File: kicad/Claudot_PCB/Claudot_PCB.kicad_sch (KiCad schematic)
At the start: 27 parts, among them SW1 SW_Push, SW10 SW_Push, SW11 SW_Push, SW12 RotaryEncoder, SW2 SW_Push, SW3 SW_Push, SW4 SW_Push, SW5 SW_Push, SW6 SW_Push, SW7 SW_Push, SW8 SW_Push, SW9 SW_Push, U1 AP2112K-3.3, U2 W25Q16JVUXIQ, U3 RP2040, Y1 Crystal_GND24

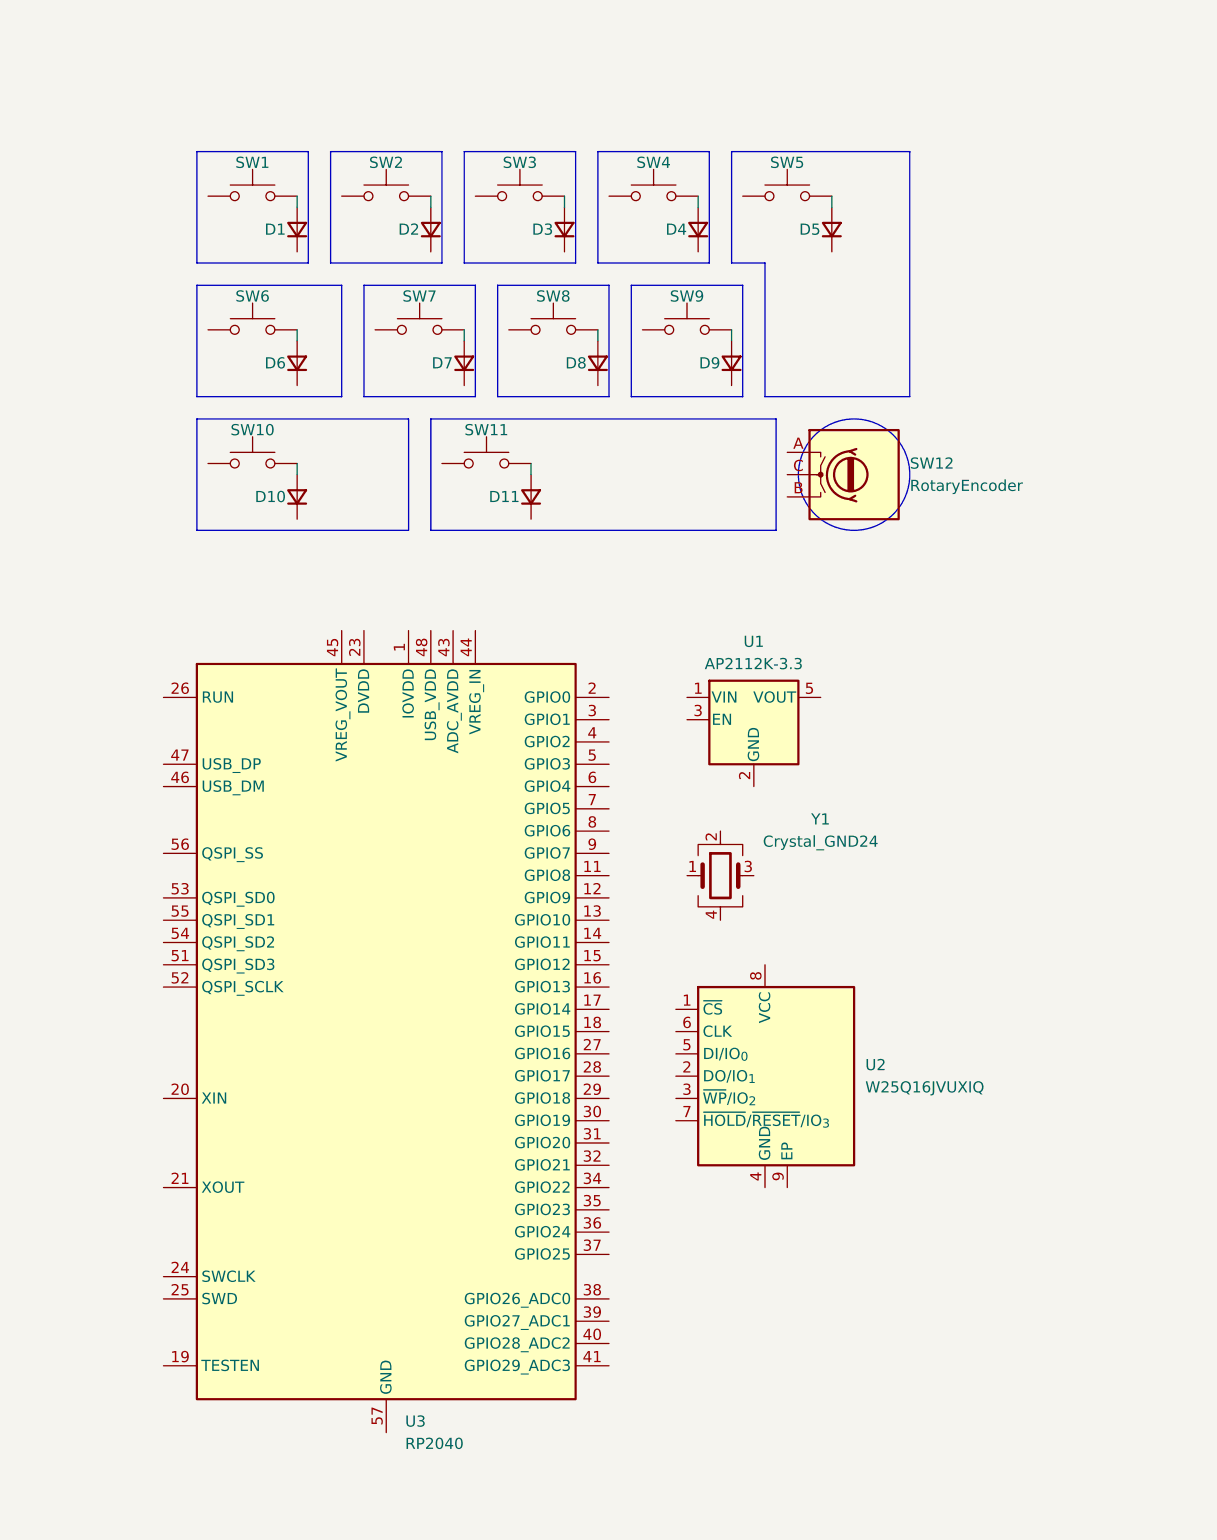
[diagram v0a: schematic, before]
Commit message: Update schematic and pcb
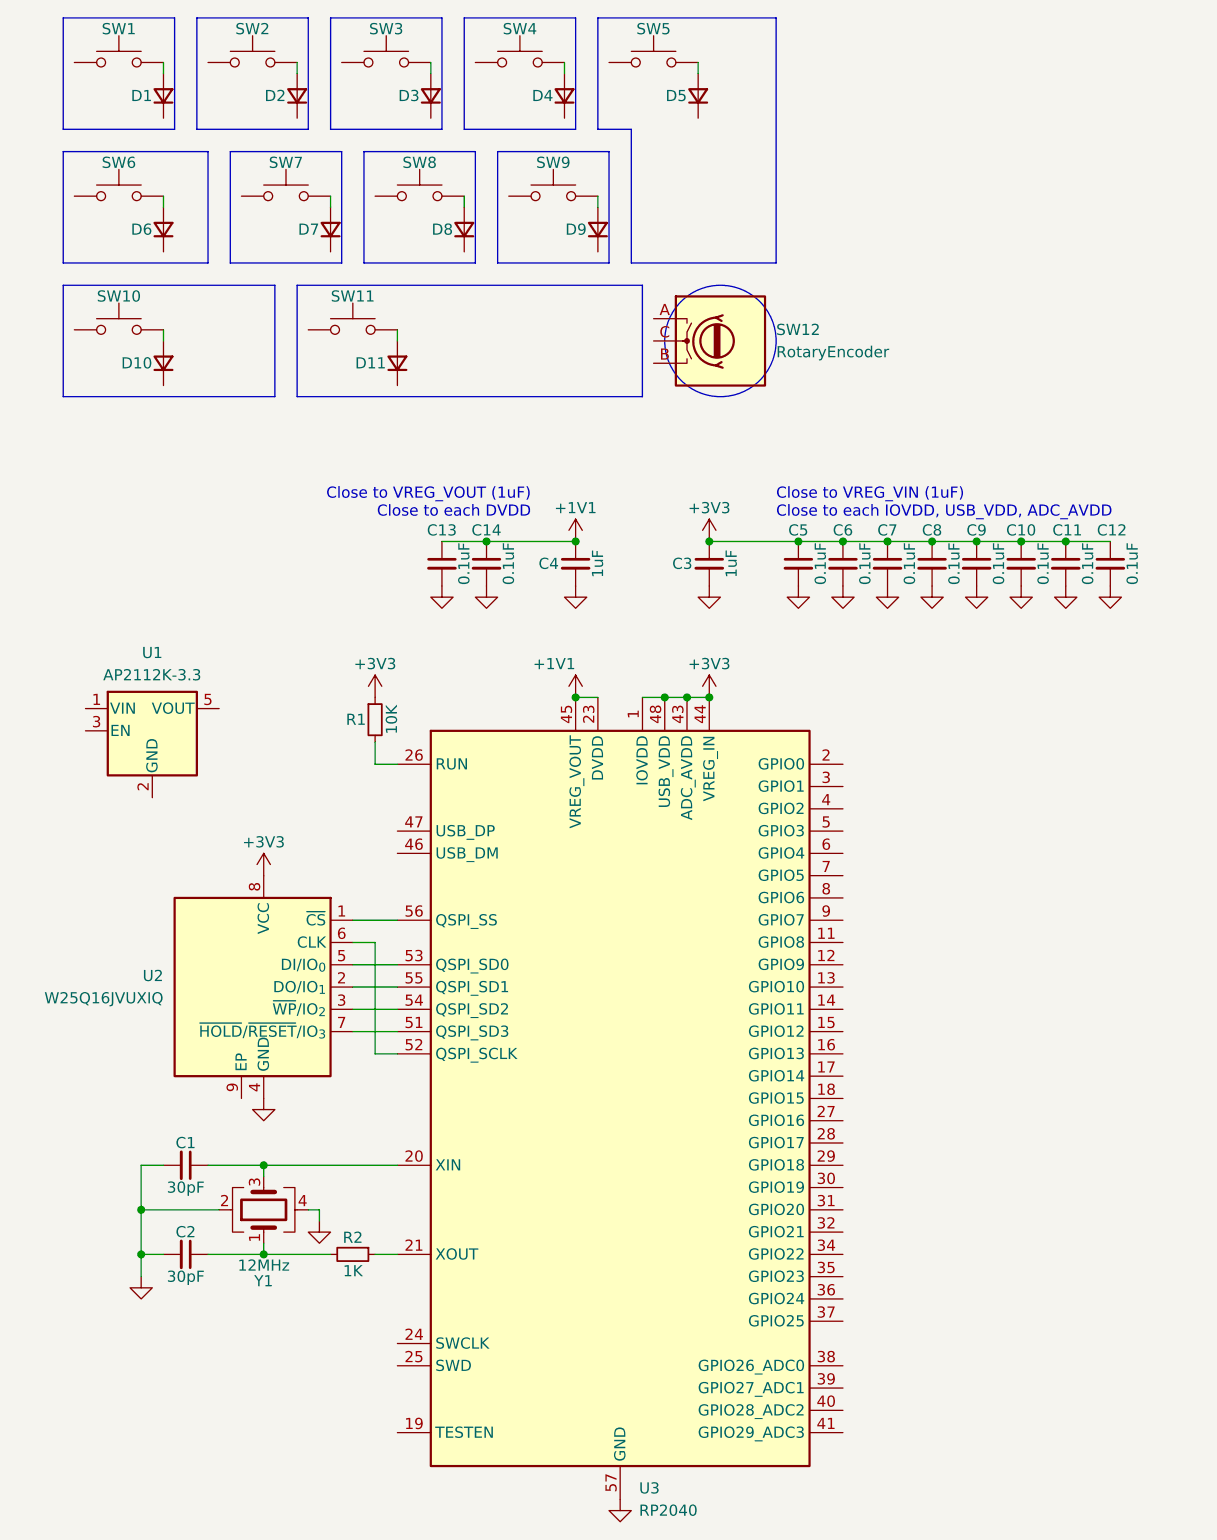
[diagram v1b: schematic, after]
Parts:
- added C1, C2: 30pF, Library:C_0402, symbol Device:C_Small
- added C10, C11, C12, C13, C14, C5, C6, C7, C8, C9: 0.1uF, Library:C_0402, symbol Device:C_Small
- added C3, C4: 1uF, Library:C_0402, symbol Device:C_Small
- added R1: 10K, Library:R_0402, symbol Device:R_Small
- added R2: 1K, Library:R_0402, symbol Device:R_Small
- Y1: value Crystal_GND24 -> 12MHz; footprint Crystal:Crystal_SMD_3225-4Pin_3.2x2.5mm -> Library:SMD3225-4P; LCSC (none) -> C9002
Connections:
- net at U2.1 (~{CS}): now also U3.56 (QSPI_SS)
- net at U2.2 (DO/IO_{1}): now also U3.55 (QSPI_SD1)
- net at U2.3 (~{WP}/IO_{2}): now also U3.54 (QSPI_SD2)
- net GND: now reaches U2.4 (GND)
- net GND: now also U3.57 (GND), Y1.2, Y1.4, C1.2, C10.2, C11.2, C12.2, C13.2, C14.2, C2.2, C3.2, C4.2, C5.2, C6.2, C7.2, C8.2, C9.2
- net at U2.5 (DI/IO_{0}): now also U3.53 (QSPI_SD0)
- net at U2.6 (CLK): now also U3.52 (QSPI_SCLK)
- net at U2.7 (~{HOLD}/~{RESET}/IO_{3}): now also U3.51 (QSPI_SD3)
- net +3V3: now reaches U2.8 (VCC)
- net +3V3: now also U3.1 (IOVDD), U3.10 (IOVDD), U3.22 (IOVDD), U3.33 (IOVDD), U3.42 (IOVDD), U3.43 (ADC_AVDD), U3.44 (VREG_IN), U3.48 (USB_VDD), U3.49 (IOVDD), C10.1, C11.1, C12.1, C3.1, C5.1, C6.1, C7.1, C8.1, C9.1, R1.1
- net at Y1.1: now also C2.1, R2.2
- net at Y1.3: now also U3.20 (XIN), C1.1
- net at U3.21 (XOUT): now also R2.1
- net +1V1: now reaches U3.23 (DVDD), U3.50 (DVDD)
- net +1V1: now also U3.45 (VREG_VOUT), C13.1, C14.1, C4.1
- net at U3.26 (RUN): now also R1.2
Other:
- note added: "Close to VREG_VIN (1uF) Close to each IOVDD, USB_VDD, ADC_AVDD"
- note added: "Close to VREG_VOUT (1uF) Close to each DVDD"
- moved on the sheet: D1, D10, D11, D2, D3, D4, D5, D6, D7, D8, D9, SW1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
